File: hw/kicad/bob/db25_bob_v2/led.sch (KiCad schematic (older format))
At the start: 35 parts, among them U20 74HC595, U21 74HC595, U24 74HC595

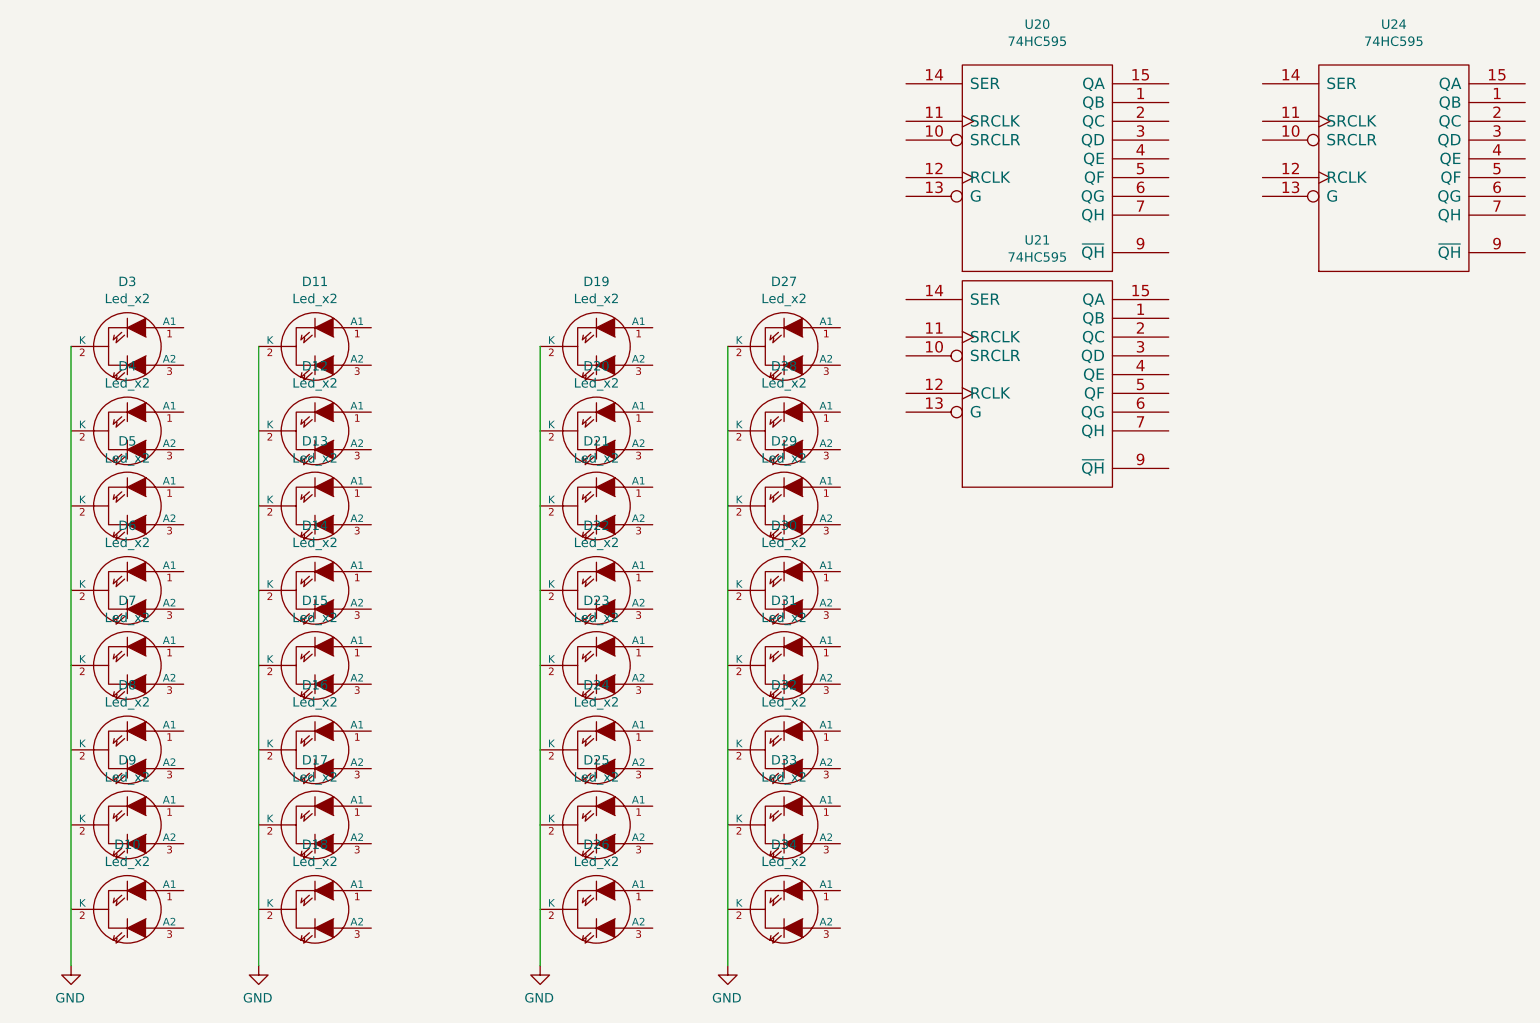
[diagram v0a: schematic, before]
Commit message: More stuff.
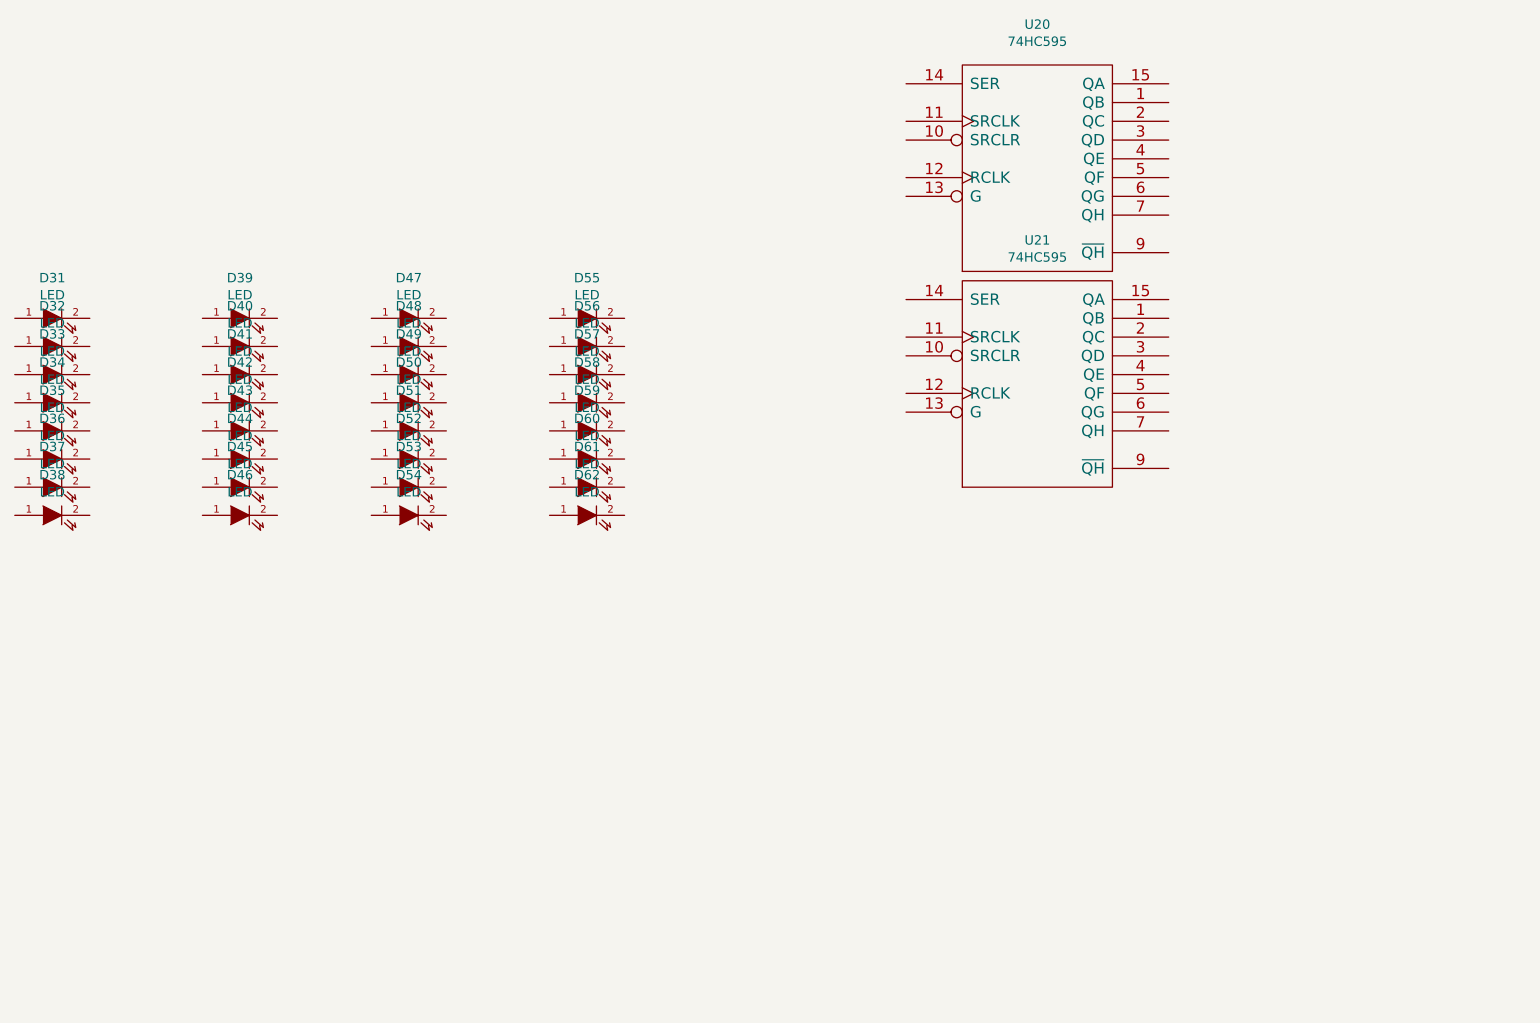
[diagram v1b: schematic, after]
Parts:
- removed D10, D11, D12, D13, D14, D15, D16, D17, D18, D19, D20, D21, D22, D23, D24, D25, D26, D27, D28, D29, D3, D30, D31, D32, D33, D34, D4, D5, D6, D7, D8, D9: Led_x2, LEDs:LED_0805, symbol Led_x2
- removed U24: 74HC595, SMD_Packages:SO-16-N, symbol 74HC595
- added D31, D32, D33, D34, D35, D36, D37, D38, D39, D40, D41, D42, D43, D44, D45, D46, D47, D48, D49, D50, D51, D52, D53, D54, D55, D56, D57, D58, D59, D60, D61, D62: LED, LEDs:LED_0603, symbol LED
